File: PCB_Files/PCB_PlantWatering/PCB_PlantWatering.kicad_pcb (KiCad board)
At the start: 4 copper layers, 109.2 x 129.5 mm, 110 parts, among them J1 Battery connection, J1 Connector to PCB2, J10 I2C Pins, J11 I2C Pins, J13 USB_C_Receptacle_USB2.0_16P, J2 AnalogSignals, J2 LED_Strip, J3 32KHZ/SQW, J3 I2C, J4 Power, J4 Solar Panel, J5 Power output, J6 Signal Sockets, J7 Connector to PCB01, J8 I2C, J9 PWR_Output, Q1 MUN5211DW1, SW1 SW_Push, SW2 SW_Push, SW3 SW_Push, SW4 SW_Push, U1 ESP32-DevKitC, U10 DS3231MZ, U11 TP4056-42-ESOP8, U12 AT24CS32-SSHM, U13 MQ-6, U14 MT3608, U2 CP2102N-Axx-xQFN28, U3 XC6220B331MR, U4 BMP280, U5 ADS1115IDGS, U6 ADS1115IDGS, U8 DW01A, U9 FS8205A

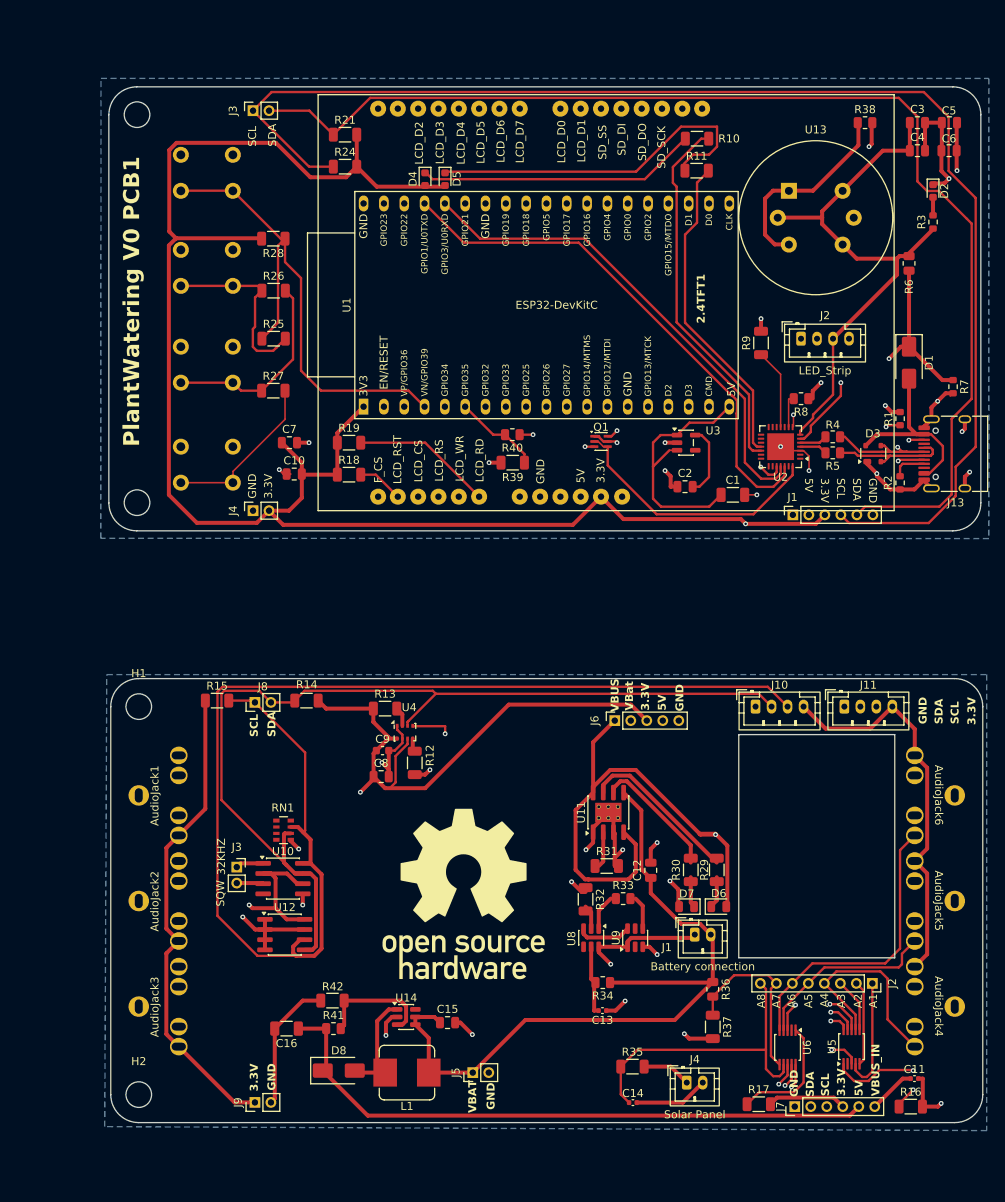
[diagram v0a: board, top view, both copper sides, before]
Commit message: added readme text
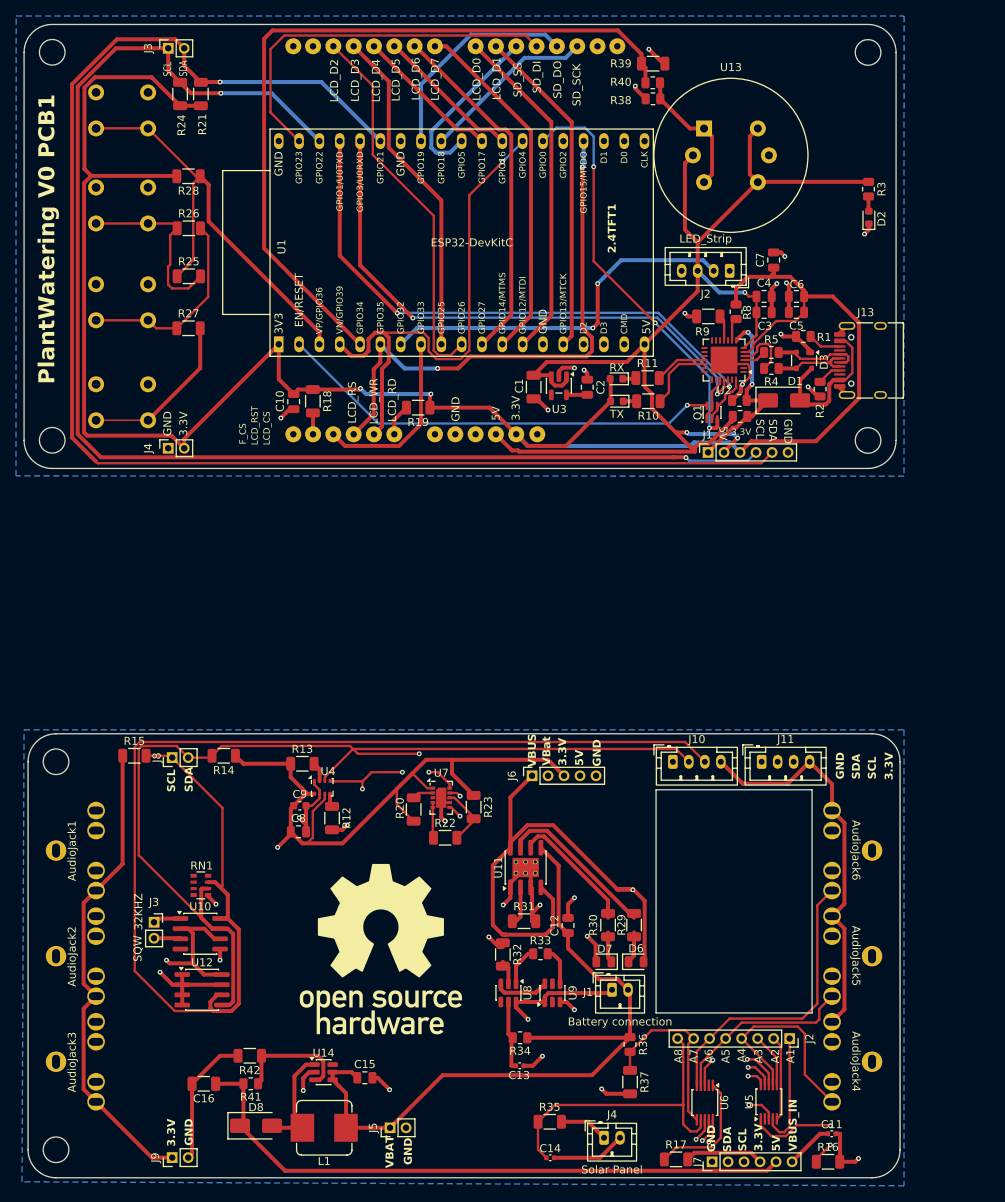
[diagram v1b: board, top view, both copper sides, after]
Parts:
- removed D4: TX, LED_SMD:LED_0603_1608Metric
- removed D5: RX, LED_SMD:LED_0603_1608Metric
- removed the H1 at (53.7, 116.0)
- removed the H2 at (53.5, 42.0)
- removed the H2 at (53.7, 164.5)
- removed the J1 at (135.5, 92.0)
- removed the J1 at (123.2, 144.5)
- removed the J2 at (145.4, 150.6)
- removed the J2 at (136.5, 70.0)
- removed the J3 at (68.0, 41.5)
- removed the J3 at (66.0, 136.1)
- removed the J4 at (122.2, 163.0)
- removed the J4 at (68.0, 91.5)
- added H1: MountingHole, MountingHole:MountingHole_3.2mm_M3, F.Cu at (144.9, 34.2)
- added H1: MountingHole, MountingHole:MountingHole_3.2mm_M3, F.Cu at (43.4, 122.9)
- added H2: MountingHole, MountingHole:MountingHole_3.2mm_M3, F.Cu at (43.4, 171.4)
- added H2: MountingHole, MountingHole:MountingHole_3.2mm_M3, F.Cu at (42.9, 34.2)
- added H4: MountingHole, MountingHole:MountingHole_3.2mm_M3, F.Cu at (144.9, 82.7)
- added J1: Battery connection, Connector_JST:JST_PH_B2B-PH-K_1x02_P2.00mm_Vertical, F.Cu at (112.9, 151.4)
- added J1: Connector to PCB2, Connector_PinSocket_2.00mm:PinSocket_1x06_P2.00mm_Vertical, F.Cu at (124.9, 84.2)
- added J2: LED_Strip, Connector_JST:JST_PH_B4B-PH-K_1x04_P2.00mm_Vertical, F.Cu at (127.6, 61.5)
- added J2: AnalogSignals, Connector_PinSocket_2.00mm:PinSocket_1x08_P2.00mm_Vertical, F.Cu at (135.1, 157.5)
- added J3: 32KHZ/SQW, Connector_PinSocket_2.00mm:PinSocket_1x02_P2.00mm_Vertical, F.Cu at (55.6, 143.0)
- added J3: I2C, Connector_PinSocket_2.00mm:PinSocket_1x02_P2.00mm_Vertical, F.Cu at (57.4, 33.7)
- added J4: Solar Panel, Connector_JST:JST_PH_B2B-PH-K_1x02_P2.00mm_Vertical, F.Cu at (111.9, 169.9)
- added J4: Power, Connector_PinSocket_2.00mm:PinSocket_1x02_P2.00mm_Vertical, F.Cu at (57.4, 83.7)
- added R20: 10k, Resistor_SMD:R_1206_3216Metric, F.Cu at (88.1, 128.9)
- added R22: 10k, Resistor_SMD:R_1206_3216Metric, F.Cu at (92.0, 132.4)
- added R23: 100k, Resistor_SMD:R_1206_3216Metric, F.Cu at (95.6, 128.6)
- added RX: RX, LED_SMD:LED_0603_1608Metric, F.Cu at (113.5, 75.0)
- added TX: TX, LED_SMD:LED_0603_1608Metric, F.Cu at (113.5, 77.8)
- added U7: CCS811, Package_LGA:AMS_LGA-10-1EP_2.7x4mm_P0.6mm, F.Cu at (91.5, 127.4)
- J7: value Connector to PCB01 -> Connector to other Board
- R1, R2, R3, R7: footprint Resistor_SMD:R_0603_1608Metric -> Resistor_SMD:R_0805_2012Metric
- moved C7 64.7 mm to (133.1, 60.2), turned to 90 degrees
- moved R39 52.9 mm to (118.0, 35.6), turned to 0 degrees
- moved R40 47.4 mm to (118.0, 38.0)
- moved R10 33.4 mm to (117.4, 77.8)
- moved C3 30.5 mm to (131.9, 66.7)
- moved C5 30.5 mm to (136.0, 66.7)
- moved R6 28.5 mm to (128.9, 79.7), turned to 0 degrees
- moved C1 28.3 mm to (103.1, 76.1), turned to -90 degrees
- moved R7 26.8 mm to (128.8, 77.7), turned to 180 degrees
- moved R38 26.7 mm to (118.0, 40.0), turned to 180 degrees
- moved R11 26.6 mm to (117.3, 74.9)
- moved C4 26.4 mm to (131.9, 64.7)
- moved C6 26.4 mm to (136.0, 64.7)
- moved R24 22.5 mm to (58.9, 39.4), turned to -90 degrees
- moved R21 18.7 mm to (61.5, 39.4), turned to -90 degrees
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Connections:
- R25 pad 1: /Analog12 -> /BUTTONS
- R28 pad 1: /Analog12 -> /BUTTONS
- R39 pad 1: /Analog10 -> /GAS_SENSOR
- R40 pad 2: /Analog10 -> /GAS_SENSOR
- SW1 pad 2: /Analog12 -> /BUTTONS
- U1 pad 10: /LCD_D3 -> /LCD_D2
- U1 pad 11: /LCD_D4 -> /LCD_D6
- U1 pad 12: /LCD_D5 -> /LCD_D7
- U1 pad 13: /LCD_D6 -> /LCD_D0
- U1 pad 15: /LCD_D7 -> /LCD_D1
- U1 pad 26: Net-(J2-Pin_2) -> /LCD_WR
- U1 pad 27: /LCD_D0 -> /LCD_D5
- U1 pad 28: /LCD_D1 -> /LCD_D4
- U1 pad 3: /Analog11 -> /BUTTONS
- U1 pad 4: /Analog12 -> /LCD_WR
- U1 pad 5: /Analog9 -> /GAS_SENSOR
- U1 pad 6: /Analog10 -> /LCD_RS
- U1 pad 7: /LCD_CS -> /LED_STRIP
- U1 pad 8: /LCD_WR -> /LCD_CS
- U1 pad 9: /LCD_D2 -> /LCD_D3
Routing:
- net /GAS_SENSOR: track 0.00 -> 95.8 mm
- net /Analog12: track 63.9 -> 0.00 mm
- net /BUTTONS: track 0.00 -> 56.4 mm
- net /RTS: track 59.3 -> 5.62 mm, vias 2 -> 0
- net Net-(U13-B1): track 69.4 -> 16.6 mm, vias 1 -> 0
- net /LED_STRIP: track 0.00 -> 46.9 mm, vias 0 -> 2
- net Net-(D5-K): track 44.7 -> 1.68 mm
- net /GPIO.0: track 46.6 -> 8.82 mm
- net /GPIO.1: track 40.0 -> 6.58 mm
- net Net-(D4-K): track 35.0 -> 1.67 mm
- net Net-(J2-Pin_2): track 33.2 -> 0.00 mm
- net /LCD_D0: track 13.2 -> 42.7 mm
- net +3.3V: track 659.9 -> 632.8 mm, vias 9 -> 8
- net /DTR: track 33.5 -> 6.56 mm
- net /VBUS_IN: track 185.3 -> 158.5 mm
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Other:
- board size 109.2 x 129.5 mm -> 109.5 x 144.2 mm
- board text added: "PlantWatering PCB01 V1"
- board text removed: "PlantWatering PCB01 V0"
